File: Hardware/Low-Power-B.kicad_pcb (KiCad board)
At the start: 2 copper layers, 55.2 x 40.6 mm, 25 parts, among them J1 USB, Q1 BC557, Q2 BC547, Q3 BC557, Q4 BC547, Q5 BC547, U1 Arduino_Pro_Micro, U2 VS1838B

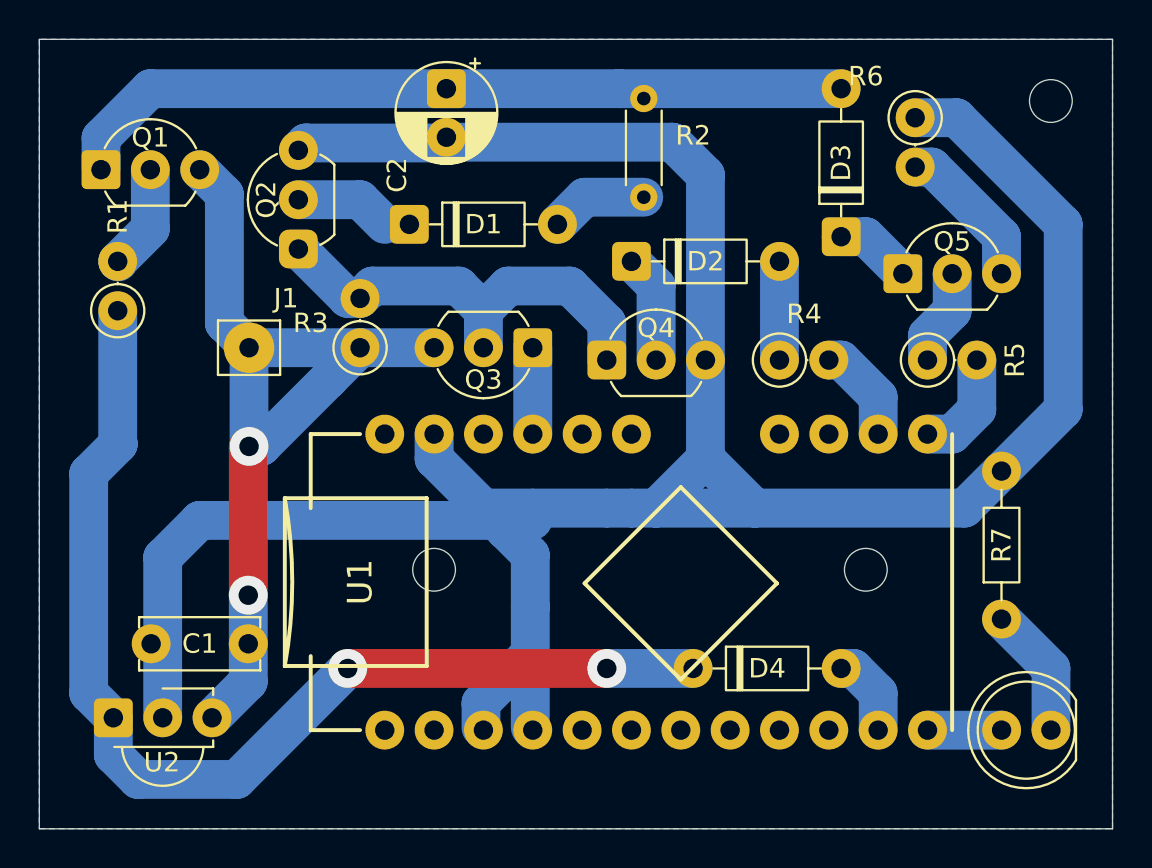
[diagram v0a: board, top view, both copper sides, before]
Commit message: update README.md
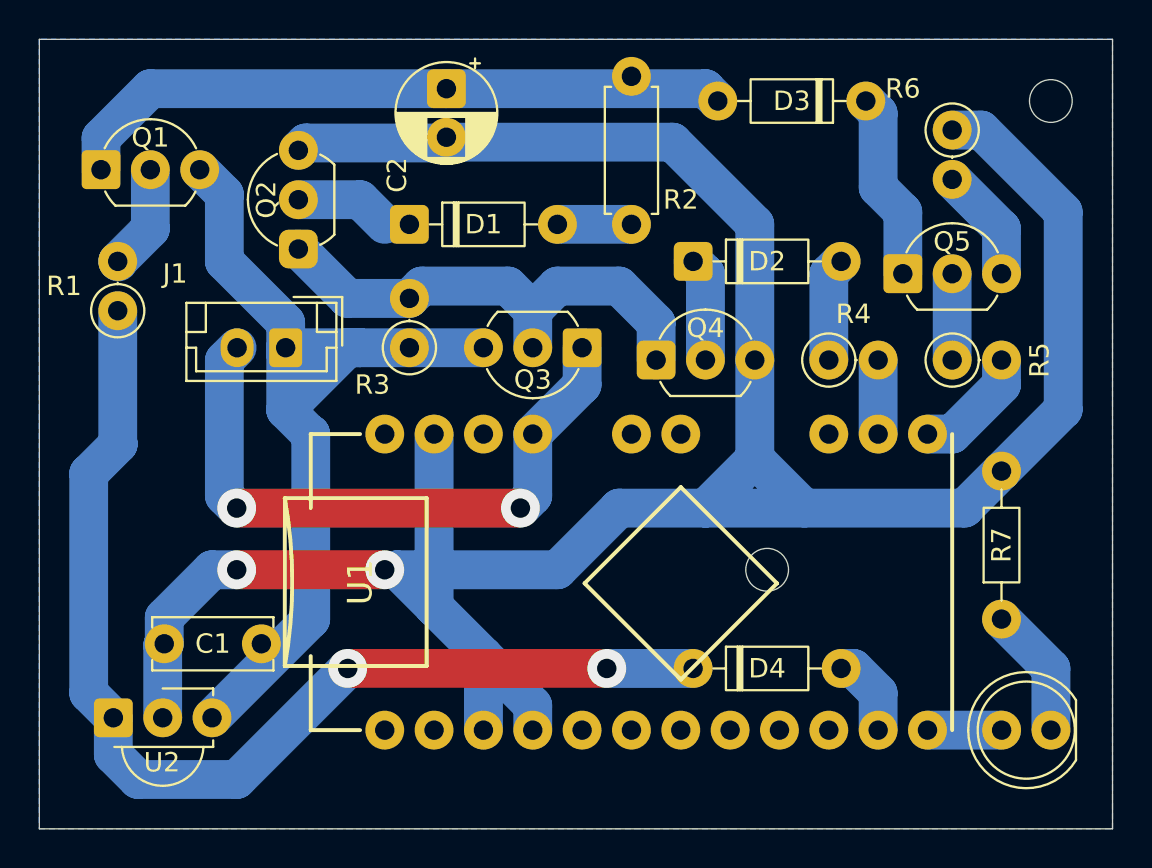
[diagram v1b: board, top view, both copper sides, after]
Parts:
- removed H3: MountingHole, MountingHole:MountingHole_2.2mm_M2_ISO7380
- J1: value USB -> USB_VBUS; footprint Connector_Pin:Pin_D1.2mm_L11.3mm_W3.0mm_Flat -> Connector_JST:JST_EH_B2B-EH-A_1x02_P2.50mm_Vertical
- R2: footprint Resistor_THT:R_Axial_DIN0204_L3.6mm_D1.6mm_P5.08mm_Horizontal -> Resistor_THT:R_Axial_DIN0207_L6.3mm_D2.5mm_P7.62mm_Horizontal
- moved H2 17.1 mm to (179.7, 78.1)
- moved D3 7.10 mm to (184.8, 54.0), turned to 180 degrees
- moved D2 3.18 mm to (175.9, 62.2)
- moved Q3 2.54 mm to (170.2, 66.7)
- moved Q4 2.54 mm to (174.0, 67.3)
- moved R3 2.54 mm to (161.3, 66.7)
- moved R4 2.54 mm to (182.9, 67.3)
- moved R6 2.01 mm to (189.2, 55.5)
- moved J1 1.88 mm to (154.9, 66.7), turned to 180 degrees
- moved R2 1.53 mm to (172.7, 60.3)
- moved R5 1.27 mm to (189.2, 67.3)
- moved C1 0.67 mm to (148.7, 81.9)
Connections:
- net +5V renamed VBUS
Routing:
- net VCC: track 4.45 -> 33.0 mm, vias 0 -> 2
- net Net-(D3-A): track 40.8 -> 34.7 mm
- net Net-(D3-K): track 3.96 -> 9.68 mm
- net GND: track 144.8 -> 141.2 mm, vias 0 -> 2
- net Net-(Q2-C): track 22.8 -> 25.4 mm
- net Net-(Q5-E): track 7.83 -> 5.91 mm
- net ON_OFF: track 5.23 -> 3.81 mm
- net Net-(D1-A): track 5.02 -> 3.81 mm
- net VBUS: track 47.4 -> 48.3 mm, vias 2 -> 0
- net DISCH: track 5.61 -> 6.13 mm
- net Net-(Q5-B): track 4.97 -> 4.45 mm
